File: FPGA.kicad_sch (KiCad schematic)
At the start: 5 parts

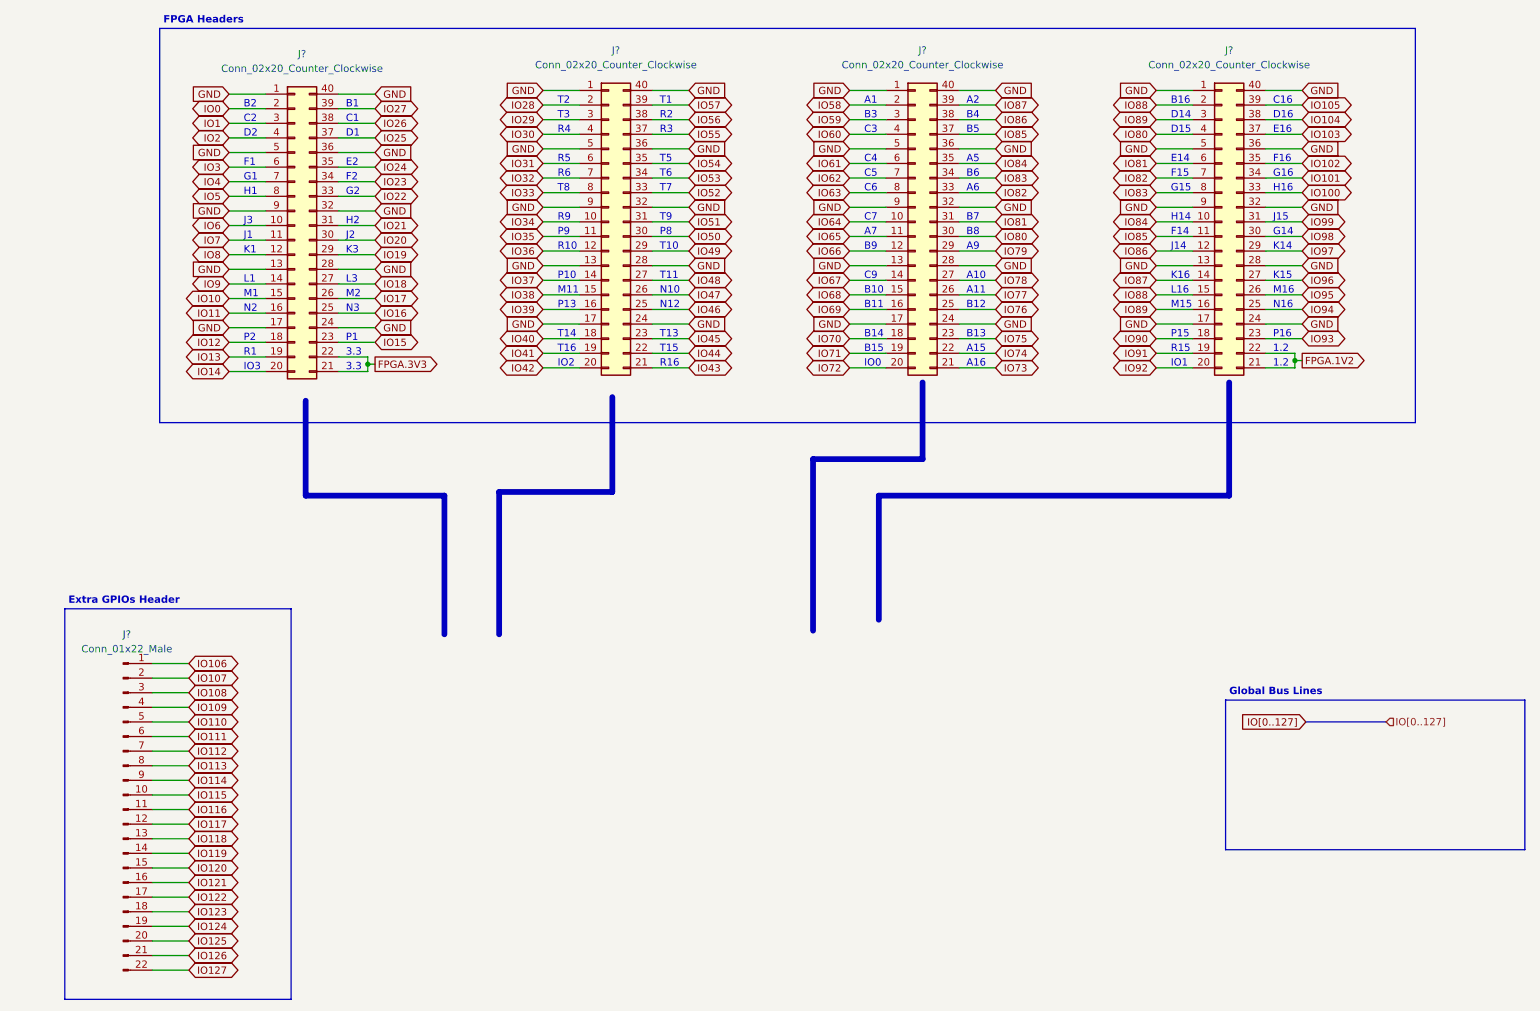
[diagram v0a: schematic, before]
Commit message: Update
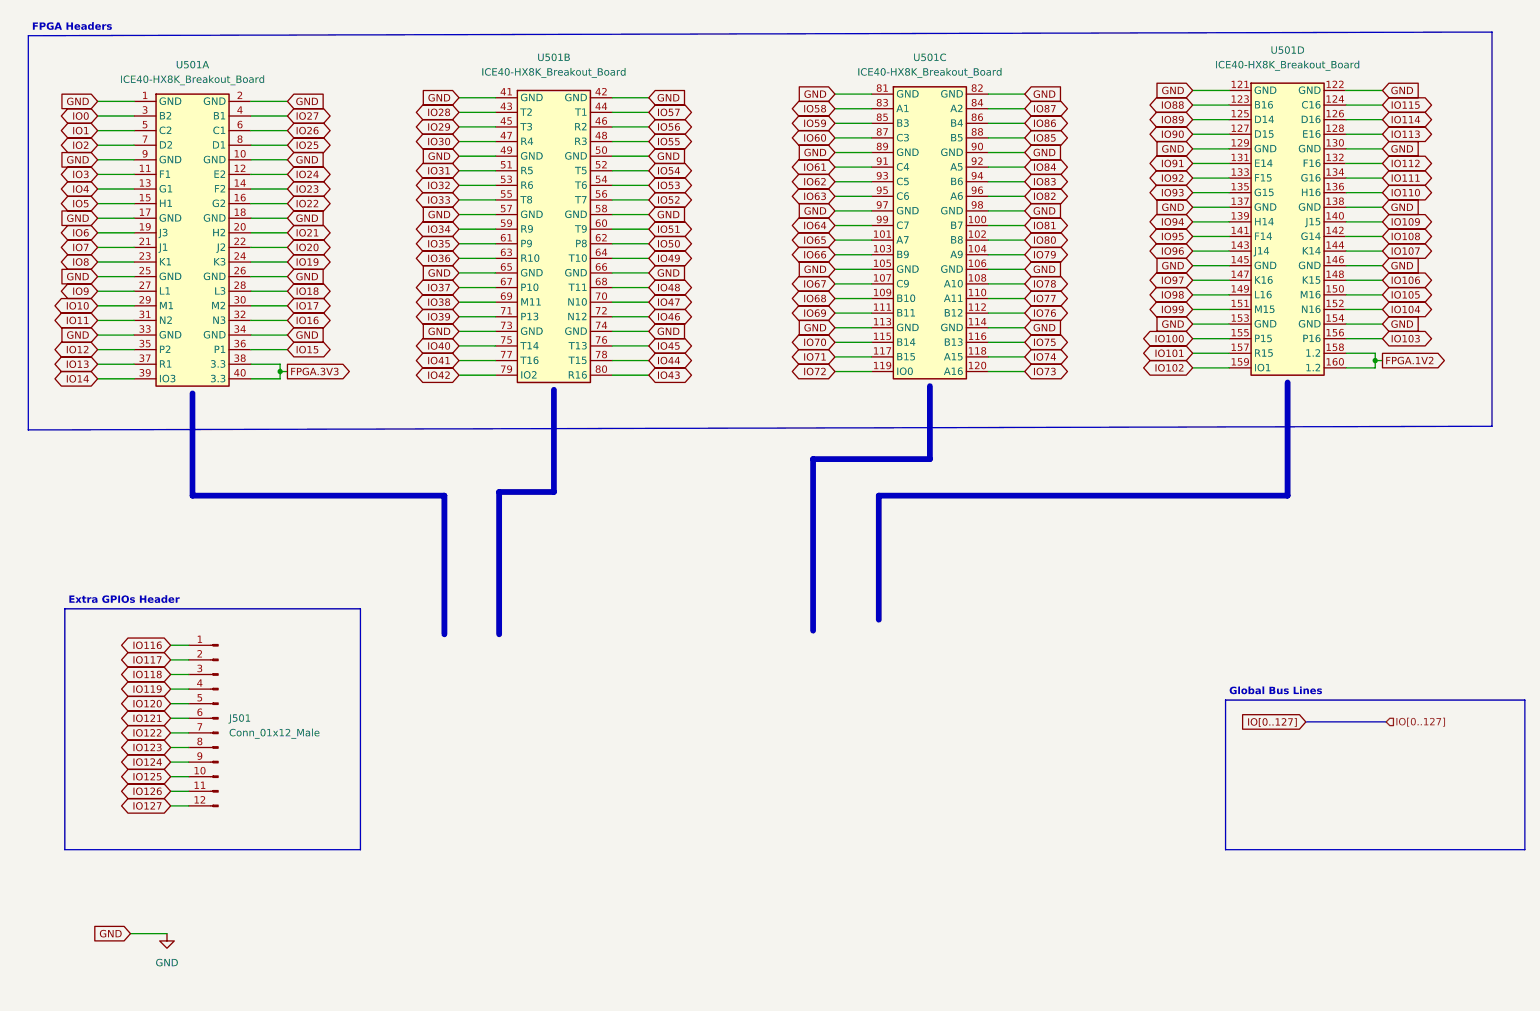
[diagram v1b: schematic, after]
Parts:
- removed J? (x4): Conn_02x20_Counter_Clockwise, symbol Connector_Generic:Conn_02x20_Counter_Clockwise
- removed J?: Conn_01x22_Male, symbol Connector:Conn_01x22_Male
- added J501: Conn_01x12_Male, Connector_PinHeader_2.54mm:PinHeader_1x12_P2.54mm_Vertical, symbol Connector:Conn_01x12_Male
- added U501: ICE40-HX8K_Breakout_Board, ECELab_Footprints:ICE40-HX8K Breakout Board, symbol ECELab_PartsLibrary:ICE40-HX8K_Breakout_Board
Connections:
- net FPGA.1V2: now also U501.158 (1.2), U501.160 (1.2)
- net FPGA.3V3: now also U501.38 (3.3), U501.40 (3.3)
- net GND: now also U501.1 (GND), U501.10 (GND), U501.105 (GND), U501.106 (GND), U501.113 (GND), U501.114 (GND), U501.121 (GND), U501.122 (GND), U501.129 (GND), U501.130 (GND), U501.137 (GND), U501.138 (GND), U501.145 (GND), U501.146 (GND), U501.153 (GND), U501.154 (GND), U501.17 (GND), U501.18 (GND), U501.2 (GND), U501.25 (GND), U501.26 (GND), U501.33 (GND), U501.34 (GND), U501.41 (GND), U501.42 (GND), U501.49 (GND), U501.50 (GND), U501.57 (GND), U501.58 (GND), U501.65 (GND), U501.66 (GND), U501.73 (GND), U501.74 (GND), U501.81 (GND), U501.82 (GND), U501.89 (GND), U501.9 (GND), U501.90 (GND), U501.97 (GND), U501.98 (GND)
- net IO0: now also U501.3 (B2)
- net IO1: now also U501.5 (C2)
- net IO10: now also U501.29 (M1)
- net IO100: now also U501.155 (P15)
- net IO101: now also U501.157 (R15)
- net IO102: now also U501.159 (IO1)
- net IO103: now also U501.156 (P16)
- net IO104: now also U501.152 (N16)
- net IO105: now also U501.150 (M16)
- net IO106: now also U501.148 (K15)
- net IO107: now also U501.144 (K14)
- net IO108: now also U501.142 (G14)
- net IO109: now also U501.140 (J15)
- net IO11: now also U501.31 (N2)
- net IO110: now also U501.136 (H16)
- net IO111: now also U501.134 (G16)
- net IO112: now also U501.132 (F16)
- net IO113: now also U501.128 (E16)
- net IO114: now also U501.126 (D16)
- net IO115: now also U501.124 (C16)
- net IO116: now also J501.1 (Pin_1)
- net IO117: now also J501.2 (Pin_2)
- net IO118: now also J501.3 (Pin_3)
- net IO119: now also J501.4 (Pin_4)
- net IO12: now also U501.35 (P2)
- net IO120: now also J501.5 (Pin_5)
- net IO121: now also J501.6 (Pin_6)
- net IO122: now also J501.7 (Pin_7)
- net IO123: now also J501.8 (Pin_8)
- net IO124: now also J501.9 (Pin_9)
- net IO125: now also J501.10 (Pin_10)
- net IO126: now also J501.11 (Pin_11)
- net IO127: now also J501.12 (Pin_12)
- net IO13: now also U501.37 (R1)
- net IO14: now also U501.39 (IO3)
- net IO15: now also U501.36 (P1)
- net IO16: now also U501.32 (N3)
- net IO17: now also U501.30 (M2)
- net IO18: now also U501.28 (L3)
- net IO19: now also U501.24 (K3)
- net IO2: now also U501.7 (D2)
- net IO20: now also U501.22 (J2)
- net IO21: now also U501.20 (H2)
- net IO22: now also U501.16 (G2)
- net IO23: now also U501.14 (F2)
- net IO24: now also U501.12 (E2)
- net IO25: now also U501.8 (D1)
- net IO26: now also U501.6 (C1)
- net IO27: now also U501.4 (B1)
- net IO28: now also U501.43 (T2)
- net IO29: now also U501.45 (T3)
- net IO3: now also U501.11 (F1)
- net IO30: now also U501.47 (R4)
- net IO31: now also U501.51 (R5)
- net IO32: now also U501.53 (R6)
- net IO33: now also U501.55 (T8)
- net IO34: now also U501.59 (R9)
- net IO35: now also U501.61 (P9)
- net IO36: now also U501.63 (R10)
- net IO37: now also U501.67 (P10)
- net IO38: now also U501.69 (M11)
- net IO39: now also U501.71 (P13)
- net IO4: now also U501.13 (G1)
- net IO40: now also U501.75 (T14)
- net IO41: now also U501.77 (T16)
- net IO42: now also U501.79 (IO2)
- net IO43: now also U501.80 (R16)
- net IO44: now also U501.78 (T15)
- net IO45: now also U501.76 (T13)
- net IO46: now also U501.72 (N12)
- net IO47: now also U501.70 (N10)
- net IO48: now also U501.68 (T11)
- net IO49: now also U501.64 (T10)
- net IO5: now also U501.15 (H1)
- net IO50: now also U501.62 (P8)
- net IO51: now also U501.60 (T9)
- net IO52: now also U501.56 (T7)
- net IO53: now also U501.54 (T6)
- net IO54: now also U501.52 (T5)
- net IO55: now also U501.48 (R3)
- net IO56: now also U501.46 (R2)
- net IO57: now also U501.44 (T1)
- net IO58: now also U501.83 (A1)
- net IO59: now also U501.85 (B3)
- net IO6: now also U501.19 (J3)
- net IO60: now also U501.87 (C3)
- net IO61: now also U501.91 (C4)
- net IO62: now also U501.93 (C5)
- net IO63: now also U501.95 (C6)
- net IO64: now also U501.99 (C7)
- net IO65: now also U501.101 (A7)
- net IO66: now also U501.103 (B9)
- net IO67: now also U501.107 (C9)
- net IO68: now also U501.109 (B10)
- net IO69: now also U501.111 (B11)
- net IO7: now also U501.21 (J1)
- net IO70: now also U501.115 (B14)
- net IO71: now also U501.117 (B15)
- net IO72: now also U501.119 (IO0)
- net IO73: now also U501.120 (A16)
- net IO74: now also U501.118 (A15)
- net IO75: now also U501.116 (B13)
- net IO76: now also U501.112 (B12)
- net IO77: now also U501.110 (A11)
- net IO78: now also U501.108 (A10)
- net IO79: now also U501.104 (A9)
- net IO8: now also U501.23 (K1)
- net IO80: now also U501.102 (B8)
- net IO81: now also U501.100 (B7)
- net IO82: now also U501.96 (A6)
- net IO83: now also U501.94 (B6)
- net IO84: now also U501.92 (A5)
- net IO85: now also U501.88 (B5)
- net IO86: now also U501.86 (B4)
- net IO87: now also U501.84 (A2)
- net IO88: now also U501.123 (B16)
- net IO89: now also U501.125 (D14)
- net IO9: now also U501.27 (L1)
- net IO90: now also U501.127 (D15)
- net IO91: now also U501.131 (E14)
- net IO92: now also U501.133 (F15)
- net IO93: now also U501.135 (G15)
- net IO94: now also U501.139 (H14)
- net IO95: now also U501.141 (F14)
- net IO96: now also U501.143 (J14)
- net IO97: now also U501.147 (K16)
- net IO98: now also U501.149 (L16)
- net IO99: now also U501.151 (M15)
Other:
- note removed: "1.2"
- note removed: "3.3"
- note removed: "A1"
- note removed: "A10"
- note removed: "A11"
- note removed: "A15"
- note removed: "A16"
- note removed: "A2"
- note removed: "A5"
- note removed: "A6"
- note removed: "A7"
- note removed: "A9"
- note removed: "B1"
- note removed: "B10"
- note removed: "B11"
- note removed: "B12"
- note removed: "B13"
- note removed: "B14"
- note removed: "B15"
- note removed: "B16"
- note removed: "B2"
- note removed: "B3"
- note removed: "B4"
- note removed: "B5"
- note removed: "B6"
- note removed: "B7"
- note removed: "B8"
- note removed: "B9"
- note removed: "C1"
- note removed: "C16"
- note removed: "C2"
- note removed: "C3"
- note removed: "C4"
- note removed: "C5"
- note removed: "C6"
- note removed: "C7"
- note removed: "C9"
- note removed: "D1"
- note removed: "D14"
- note removed: "D15"
- note removed: "D16"
- note removed: "D2"
- note removed: "E14"
- note removed: "E16"
- note removed: "E2"
- note removed: "F1"
- note removed: "F14"
- note removed: "F15"
- note removed: "F16"
- note removed: "F2"
- note removed: "G1"
- note removed: "G14"
- note removed: "G15"
- note removed: "G16"
- note removed: "G2"
- note removed: "H1"
- note removed: "H14"
- note removed: "H16"
- note removed: "H2"
- note removed: "IO0"
- note removed: "IO1"
- note removed: "IO2"
- note removed: "IO3"
- note removed: "J1"
- note removed: "J14"
- note removed: "J15"
- note removed: "J2"
- note removed: "J3"
- note removed: "K1"
- note removed: "K14"
- note removed: "K15"
- note removed: "K16"
- note removed: "K3"
- note removed: "L1"
- note removed: "L16"
- note removed: "L3"
- note removed: "M1"
- note removed: "M11"
- note removed: "M15"
- note removed: "M16"
- note removed: "M2"
- note removed: "N10"
- note removed: "N12"
- note removed: "N16"
- note removed: "N2"
- note removed: "N3"
- note removed: "P1"
- note removed: "P10"
- note removed: "P13"
- note removed: "P15"
- note removed: "P16"
- note removed: "P2"
- note removed: "P8"
- note removed: "P9"
- note removed: "R1"
- note removed: "R10"
- note removed: "R15"
- note removed: "R16"
- note removed: "R2"
- note removed: "R3"
- note removed: "R4"
- note removed: "R5"
- note removed: "R6"
- note removed: "R9"
- note removed: "T1"
- note removed: "T10"
- note removed: "T11"
- note removed: "T13"
- note removed: "T14"
- note removed: "T15"
- note removed: "T16"
- note removed: "T2"
- note removed: "T3"
- note removed: "T5"
- note removed: "T6"
- note removed: "T7"
- note removed: "T8"
- note removed: "T9"

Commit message: Complete Draft 1 of PCB Design
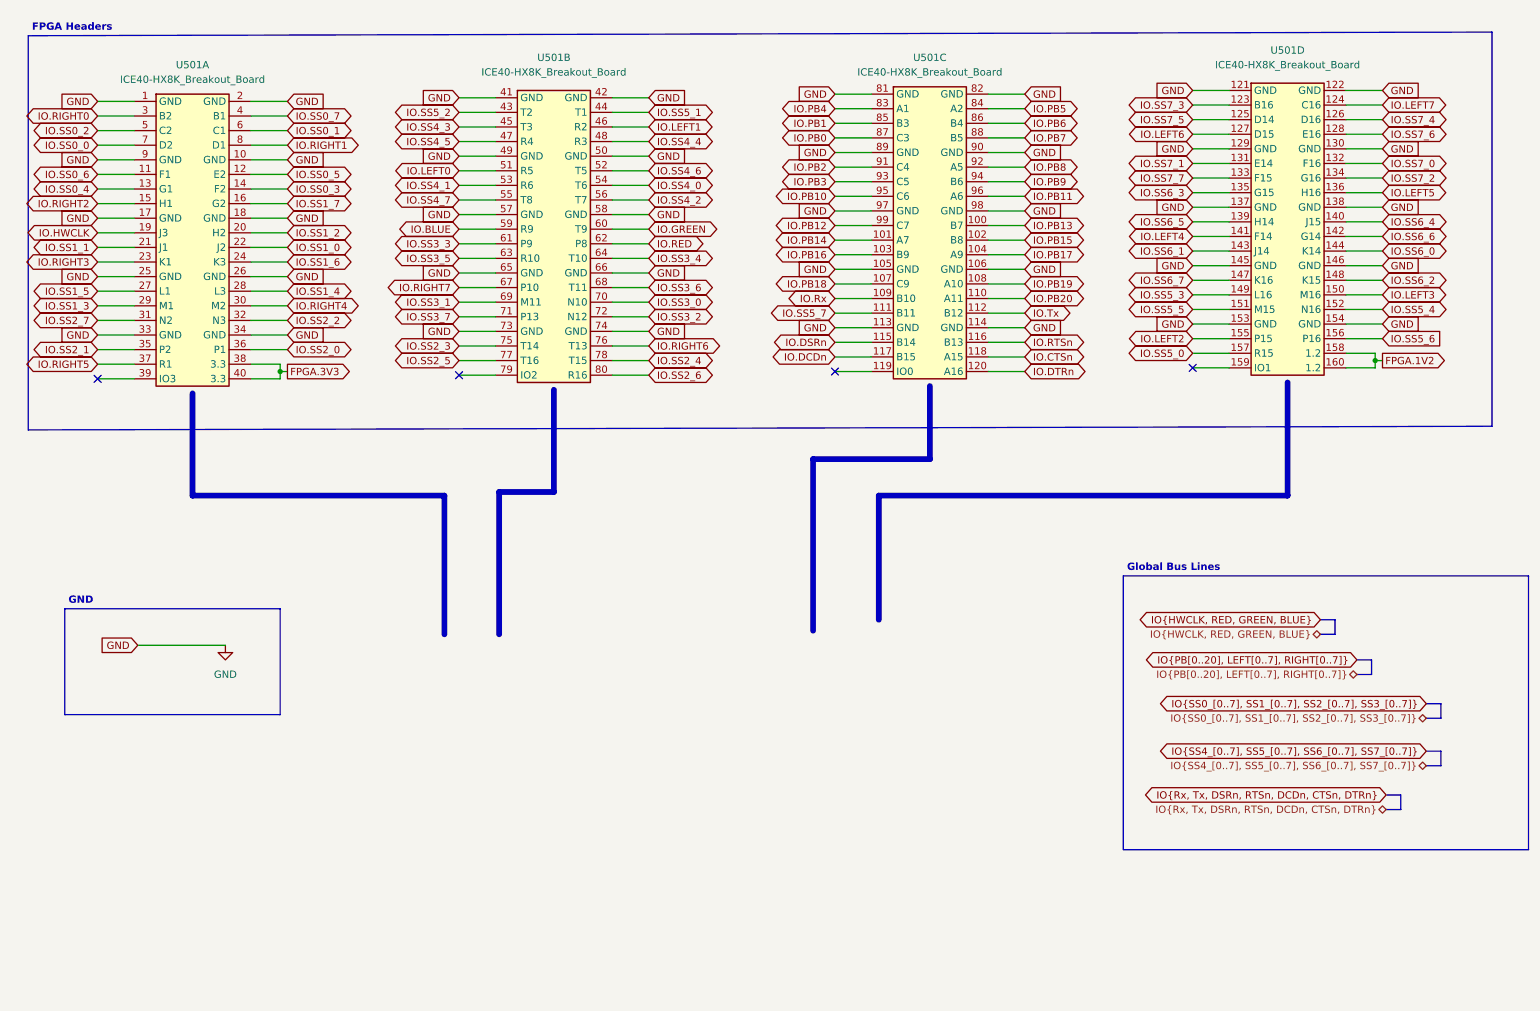
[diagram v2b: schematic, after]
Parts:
- removed J501: Conn_01x12_Male, Connector_PinHeader_2.54mm:PinHeader_1x12_P2.54mm_Vertical, symbol Connector:Conn_01x12_Male
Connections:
- net IO0 renamed IO.RIGHT0
- net IO1 renamed IO.SS0_2
- net IO10 renamed IO.SS1_3
- net IO100 renamed IO.LEFT2
- net IO101 renamed IO.SS5_0
- net IO102: no longer names the net of U501.159 (IO1)
- net IO103 renamed IO.SS5_6
- net IO104 renamed IO.SS5_4
- net IO105 renamed IO.LEFT3
- net IO106 renamed IO.SS6_2
- net IO107 renamed IO.SS6_0
- net IO108 renamed IO.SS6_6
- net IO109 renamed IO.SS6_4
- net IO11 renamed IO.SS2_7
- net IO110 renamed IO.LEFT5
- net IO111 renamed IO.SS7_2
- net IO112 renamed IO.SS7_0
- net IO113 renamed IO.SS7_6
- net IO114 renamed IO.SS7_4
- net IO115 renamed IO.LEFT7
- net IO12 renamed IO.SS2_1
- net IO13 renamed IO.RIGHT5
- net IO14: no longer names the net of U501.39 (IO3)
- net IO15 renamed IO.SS2_0
- net IO16 renamed IO.SS2_2
- net IO17 renamed IO.RIGHT4
- net IO18 renamed IO.SS1_4
- net IO19 renamed IO.SS1_6
- net IO2 renamed IO.SS0_0
- net IO20 renamed IO.SS1_0
- net IO21 renamed IO.SS1_2
- net IO22 renamed IO.SS1_7
- net IO23 renamed IO.SS0_3
- net IO24 renamed IO.SS0_5
- net IO25 renamed IO.RIGHT1
- net IO26 renamed IO.SS0_1
- net IO27 renamed IO.SS0_7
- net IO28 renamed IO.SS5_2
- net IO29 renamed IO.SS4_3
- net IO3 renamed IO.SS0_6
- net IO30 renamed IO.SS4_5
- net IO31 renamed IO.LEFT0
- net IO32 renamed IO.SS4_1
- net IO33 renamed IO.SS4_7
- net IO34 renamed IO.BLUE
- net IO35 renamed IO.SS3_3
- net IO36 renamed IO.SS3_5
- net IO37 renamed IO.RIGHT7
- net IO38 renamed IO.SS3_1
- net IO39 renamed IO.SS3_7
- net IO4 renamed IO.SS0_4
- net IO40 renamed IO.SS2_3
- net IO41 renamed IO.SS2_5
- net IO42: no longer names the net of U501.79 (IO2)
- net IO43 renamed IO.SS2_6
- net IO44 renamed IO.SS2_4
- net IO45 renamed IO.RIGHT6
- net IO46 renamed IO.SS3_2
- net IO47 renamed IO.SS3_0
- net IO48 renamed IO.SS3_6
- net IO49 renamed IO.SS3_4
- net IO5 renamed IO.RIGHT2
- net IO50 renamed IO.RED
- net IO51 renamed IO.GREEN
- net IO52 renamed IO.SS4_2
- net IO53 renamed IO.SS4_0
- net IO54 renamed IO.SS4_6
- net IO55 renamed IO.SS4_4
- net IO56 renamed IO.LEFT1
- net IO57 renamed IO.SS5_1
- net IO58 renamed IO.PB4
- net IO59 renamed IO.PB1
- net IO6 renamed IO.HWCLK
- net IO60 renamed IO.PB0
- net IO61 renamed IO.PB2
- net IO62 renamed IO.PB3
- net IO63 renamed IO.PB10
- net IO64 renamed IO.PB12
- net IO65 renamed IO.PB14
- net IO66 renamed IO.PB16
- net IO67 renamed IO.PB18
- net IO68 renamed IO.Rx
- net IO69 renamed IO.SS5_7
- net IO7 renamed IO.SS1_1
- net IO70 renamed IO.DSRn
- net IO71 renamed IO.DCDn
- net IO72: no longer names the net of U501.119 (IO0)
- net IO73 renamed IO.DTRn
- net IO74 renamed IO.CTSn
- net IO75 renamed IO.RTSn
- net IO76 renamed IO.Tx
- net IO77 renamed IO.PB20
- net IO78 renamed IO.PB19
- net IO79 renamed IO.PB17
- net IO8 renamed IO.RIGHT3
- net IO80 renamed IO.PB15
- net IO81 renamed IO.PB13
- net IO82 renamed IO.PB11
- net IO83 renamed IO.PB9
- net IO84 renamed IO.PB8
- net IO85 renamed IO.PB7
- net IO86 renamed IO.PB6
- net IO87 renamed IO.PB5
- net IO88 renamed IO.SS7_3
- net IO89 renamed IO.SS7_5
- net IO9 renamed IO.SS1_5
- net IO90 renamed IO.LEFT6
- net IO91 renamed IO.SS7_1
- net IO92 renamed IO.SS7_7
- net IO93 renamed IO.SS6_3
- net IO94 renamed IO.SS6_5
- net IO95 renamed IO.LEFT4
- net IO96 renamed IO.SS6_1
- net IO97 renamed IO.SS6_7
- net IO98 renamed IO.SS5_3
- net IO99 renamed IO.SS5_5
- no-connect marks 0 -> 4
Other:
- note added: "GND"
- note removed: "Extra GPIOs Header"
